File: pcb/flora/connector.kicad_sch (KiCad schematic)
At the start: 9 parts, among them J1 KF350-3.5-2P, J2 KF350-3.5-2P, J3 KF350-3.5-2P, J4 10118193-0001LF, J5 PH-2V, U3 USBLC6-2P6

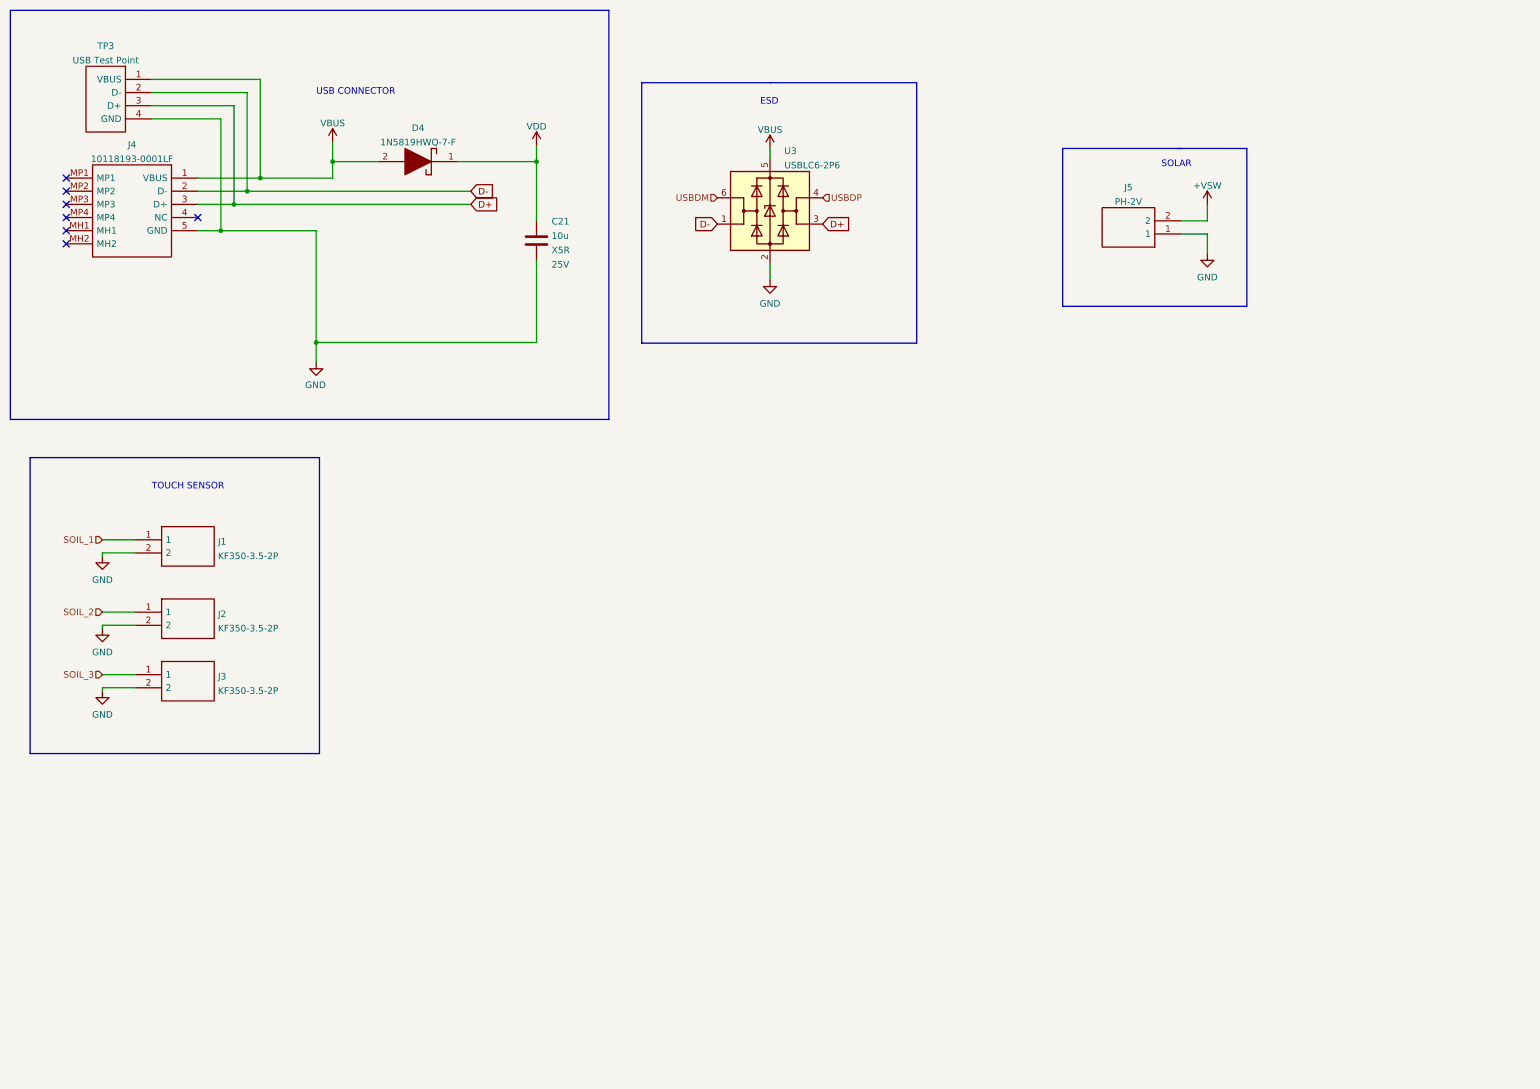
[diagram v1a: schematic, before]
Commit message: released Rev A
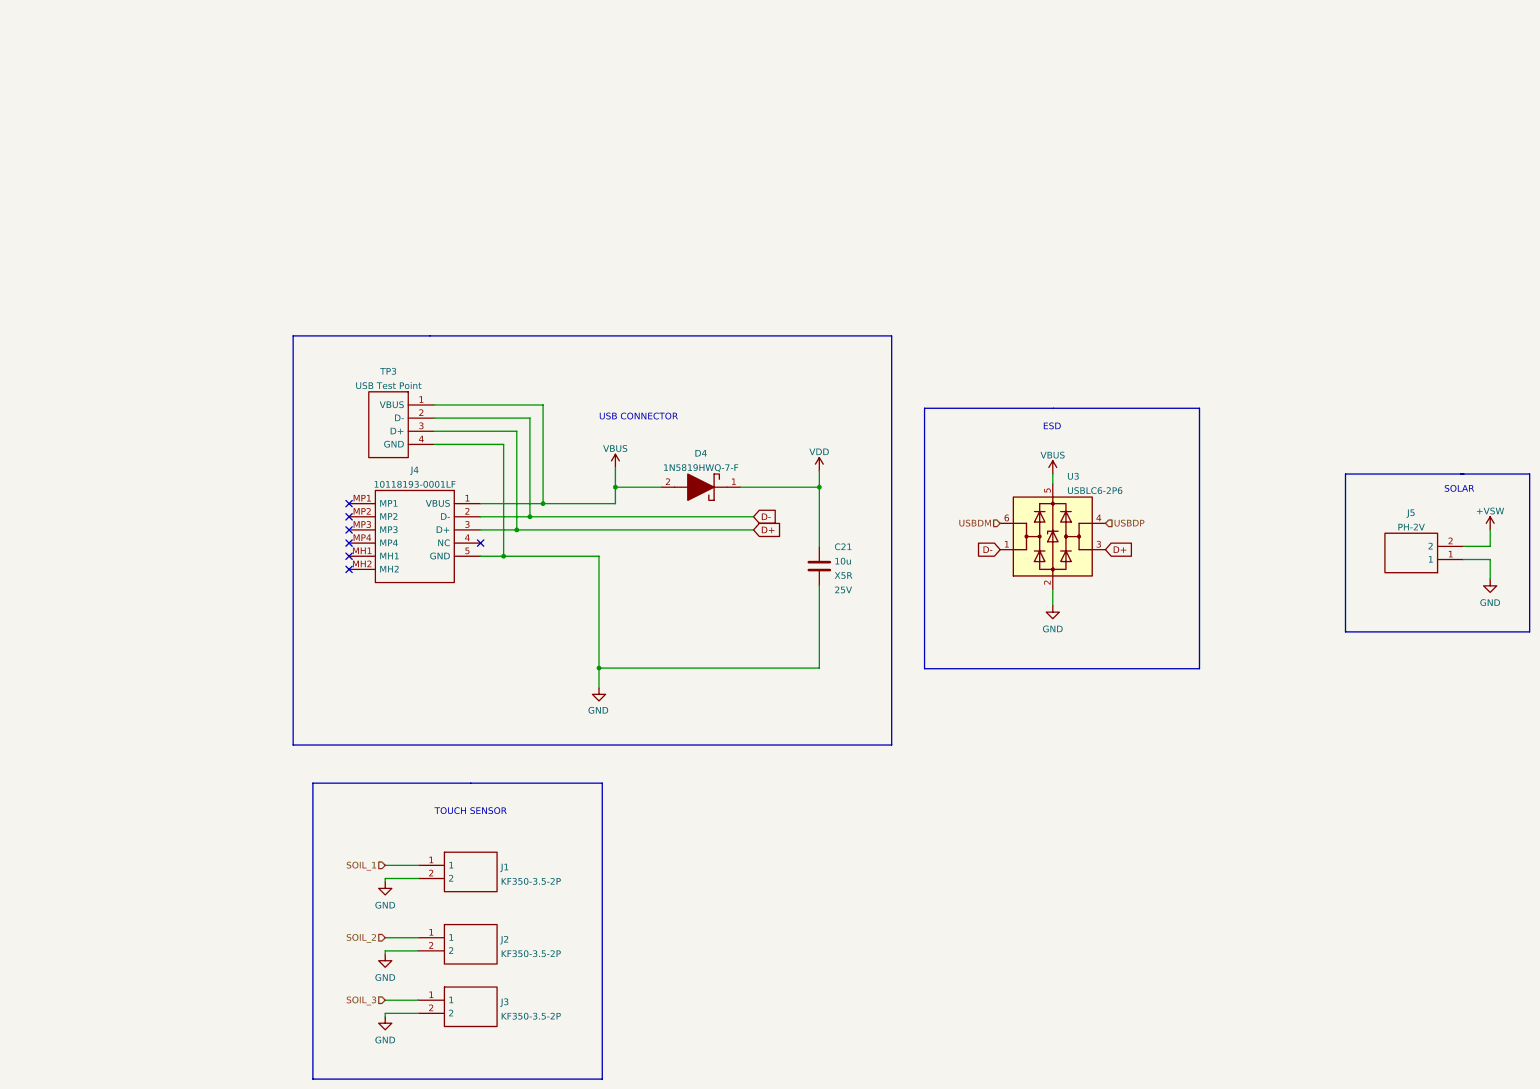
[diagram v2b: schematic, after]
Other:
- moved on the sheet: C21, D4, J1, J2, J3, J4, J5, TP3, U3

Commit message: added image
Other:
- title: (none) -> FLORA
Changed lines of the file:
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@@
 (kicad_sch (version 20211123) (generator eeschema)
   (paper "A3")
+  (title_block
+    (title "FLORA")
+    (date "2022-06-01")
+    (rev "B")
+  )
   (junction (at 123.825 116.84) (diameter 0) (color 0 0 0 0)
   )

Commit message: Finished schematic for RA-01 design
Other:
- title: FLORA -> FLORA-RA01H
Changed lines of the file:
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@@
   (paper "A3")
   (title_block
-    (title "FLORA")
-    (date "2022-07-01")
+    (title "FLORA-RA01H")
+    (date "2022-12-05")
     (rev "C")
   )
